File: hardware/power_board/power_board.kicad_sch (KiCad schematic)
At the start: 2 parts, among them J1 MCU, J9 MAINS_IN

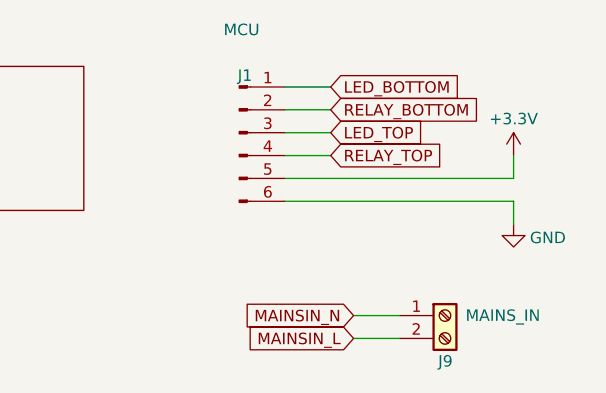
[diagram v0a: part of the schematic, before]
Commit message: v2 Boards for fabrication
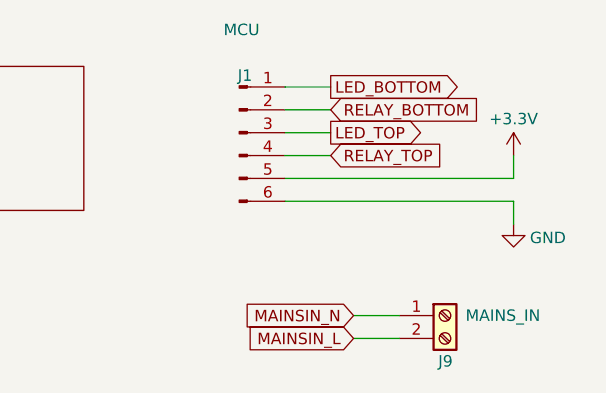
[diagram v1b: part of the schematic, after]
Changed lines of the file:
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@@
     )
   )
-  (global_label "LED_BOTTOM" (shape input) (at 162.56 43.18 0) (fields_autoplaced)
+  (global_label "LED_BOTTOM" (shape output) (at 162.56 43.18 0) (fields_autoplaced)
     (effects (font (size 1.27 1.27)) (justify left))
     (property "Intersheetrefs" "${INTERSHEET_REFS}" (at 177.2775 43.18 0)
@@
     )
   )
-  (global_label "LED_TOP" (shape input) (at 162.56 48.26 0) (fields_autoplaced)
+  (global_label "LED_TOP" (shape output) (at 162.56 48.26 0) (fields_autoplaced)
     (effects (font (size 1.27 1.27)) (justify left))
     (property "Intersheetrefs" "${INTERSHEET_REFS}" (at 173.528 48.26 0)
